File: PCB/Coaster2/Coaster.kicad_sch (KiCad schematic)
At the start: 409 parts

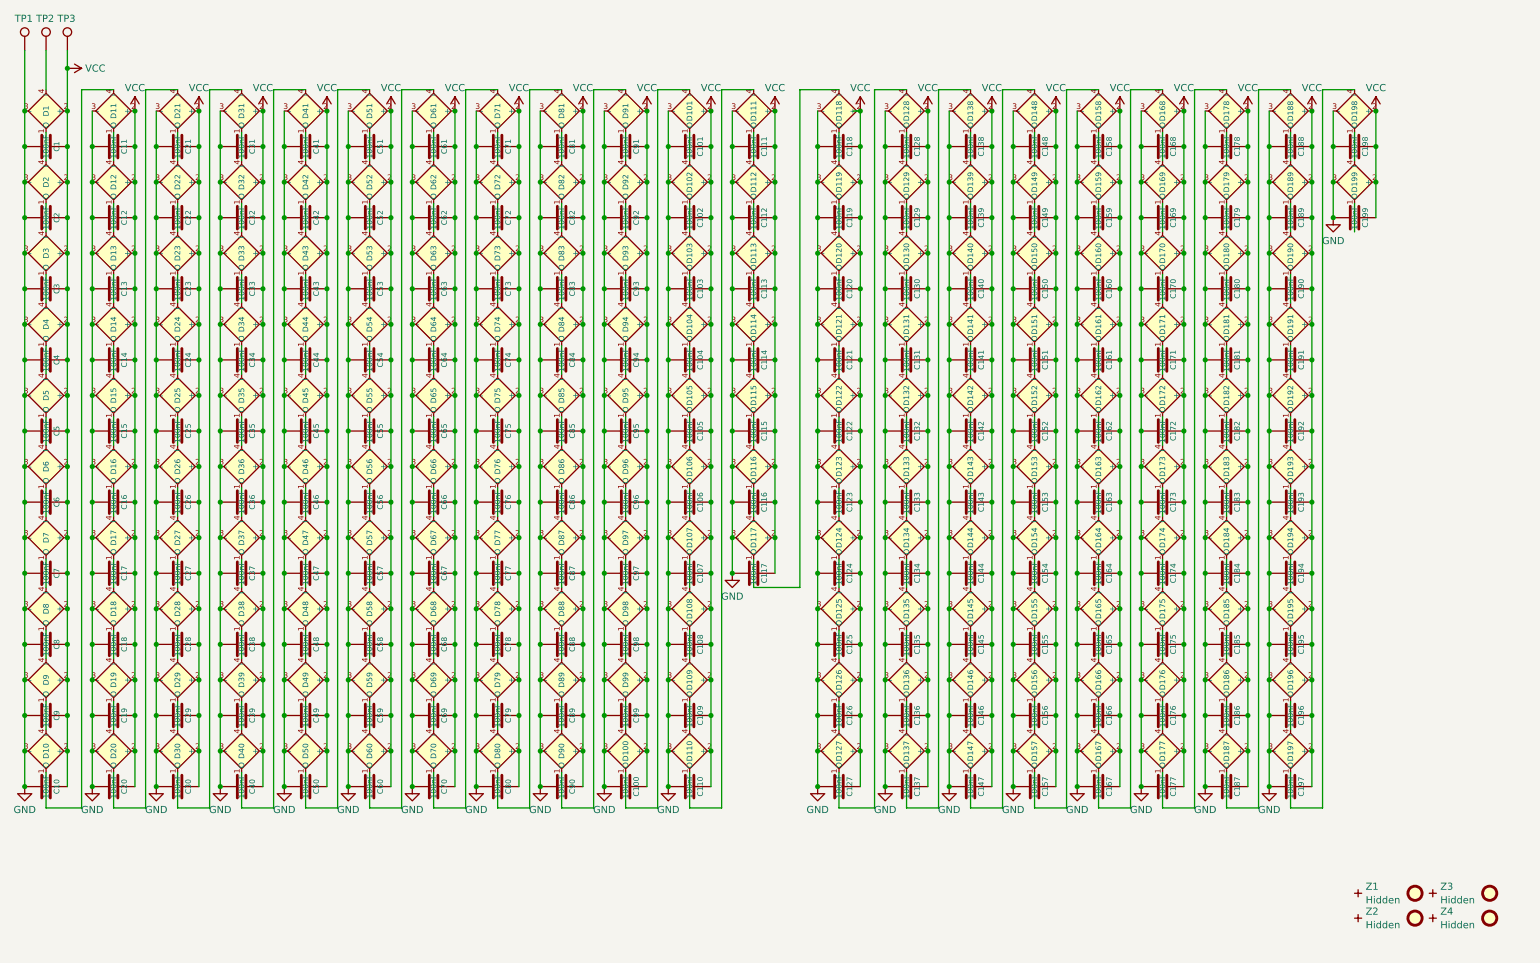
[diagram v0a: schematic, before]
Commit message: Tracked
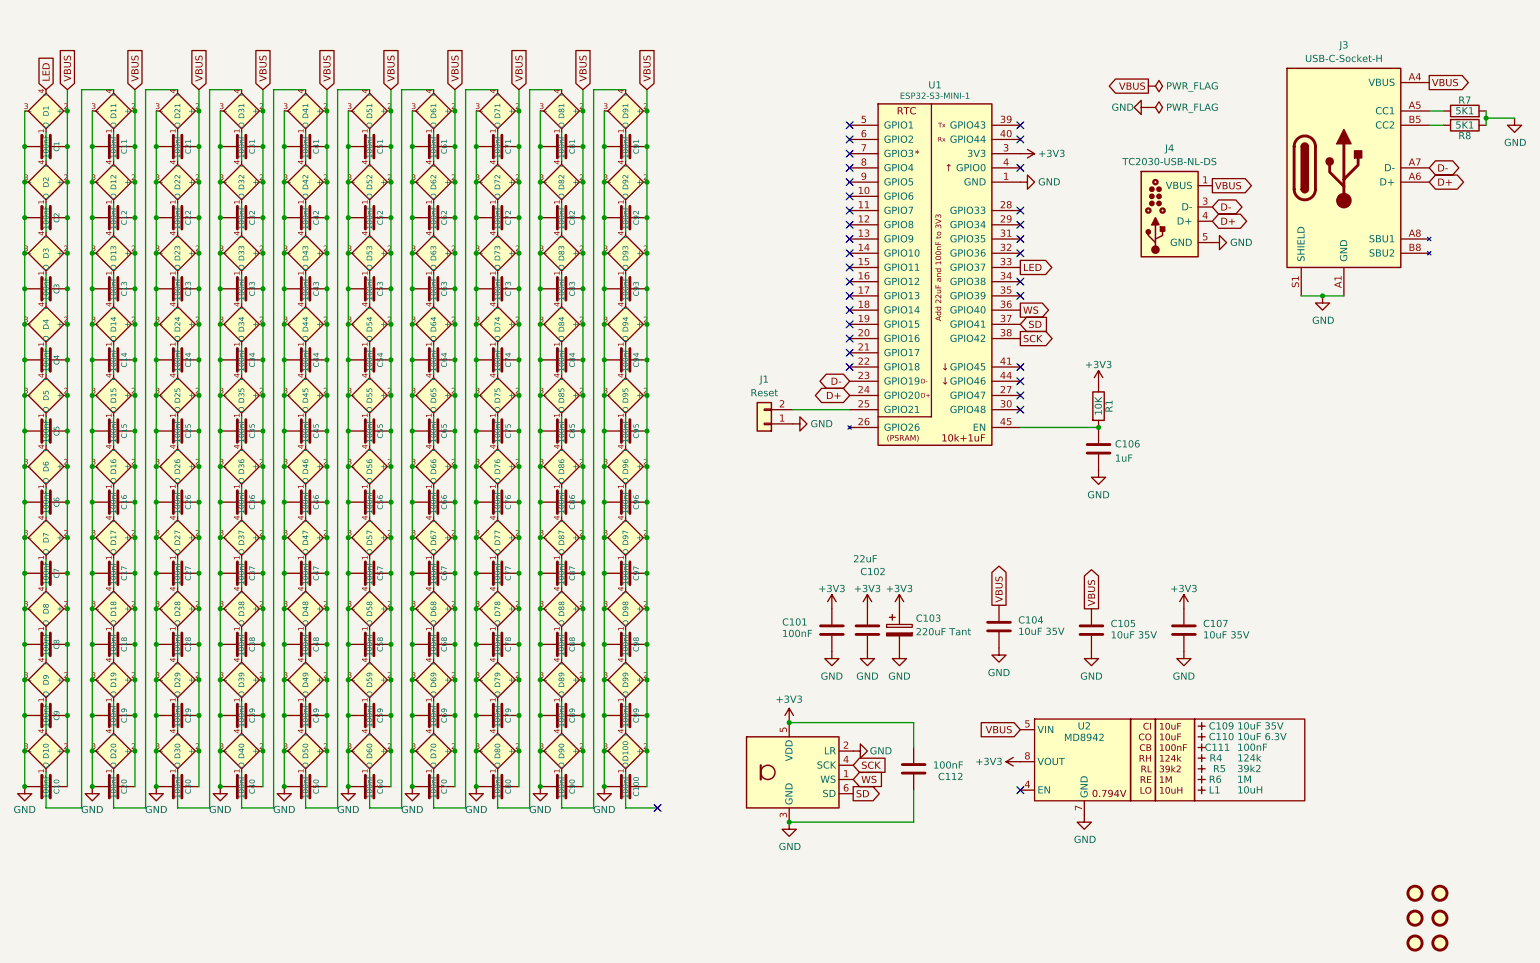
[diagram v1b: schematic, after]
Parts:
- removed C103, C108, C109, C110, C111, C113, C114, C115, C116, C117, C118, C119, C120, C121, C122, C123, C124, C125, C126, C127, C128, C129, C130, C131, C132, C133, C134, C135, C136, C137, C138, C139, C140, C141, C142, C143, C144, C145, C146, C147, C148, C149, C150, C151, C152, C153, C154, C155, C156, C157, C158, C159, C160, C161, C162, C163, C164, C165, C166, C167, C168, C169, C170, C171, C172, C173, C174, C175, C176, C177, C178, C179, C180, C181, C182, C183, C184, C185, C186, C187, C188, C189, C190, C191, C192, C193, C194, C195, C196, C197, C198, C199: 100nF, RevK:C_0402, symbol Device:C
- removed D101, D102, D103, D104, D105, D106, D107, D108, D109, D110, D111, D112, D113, D114, D115, D116, D117, D118, D119, D120, D121, D122, D123, D124, D125, D126, D127, D128, D129, D130, D131, D132, D133, D134, D135, D136, D137, D138, D139, D140, D141, D142, D143, D144, D145, D146, D147, D148, D149, D150, D151, D152, D153, D154, D155, D156, D157, D158, D159, D160, D161, D162, D163, D164, D165, D166, D167, D168, D169, D170, D171, D172, D173, D174, D175, D176, D177, D178, D179, D180, D181, D182, D183, D184, D185, D186, D187, D188, D189, D190, D191, D192, D193, D194, D195, D196, D197, D198, D199: XL-1010RGBC-WS2812B, RevK:SMD1010, symbol RevK:WS2812B-1mm
- removed TP1: GND, RevK:Round, symbol Connector:TestPoint
- removed TP2: DIN, RevK:Round, symbol Connector:TestPoint
- removed TP3: PWR, RevK:Round, symbol Connector:TestPoint
- removed Z1, Z2, Z3, Z4: Hidden, RevK:PCB-Join1, symbol RevK:Hidden
- added C103: 220uF Tant, RevK:CP_EIA-3528-21_Kemet-B, symbol Device:C_Polarized
- added C109: 10uF 35V, RevK:C_0603_, symbol RevK:Hidden
- added C110: 10uF 6.3V, RevK:C_0603_, symbol RevK:Hidden
- added C111: 100nF, RevK:C_0603_, symbol RevK:Hidden
- added FID5: Fiducial, RevK:Hole-Tooling, symbol Mechanical:Fiducial
- added FID6: Fiducial, Fiducial:Fiducial_1mm_Mask2mm, symbol Mechanical:Fiducial
- added J1: Reset, RevK:AA-Pad, symbol Connector_Generic:Conn_01x02
- added J3: USB-C-Socket-H, RevK:USB-C-Socket-H, symbol RevK:USB-C-Socket-H
- added J4: TC2030-USB-NL-DS, RevK:Tag-Connect_TC2030-IDC-NL_2x03_P1.27mm_Vertical, symbol RevK:TC2030-USB-NL
- added L1: 10uH, RevK:L_4x4_, symbol RevK:Hidden
- added R1: 10K, RevK:R_0402, symbol Device:R
- added R4: 124k, RevK:R_0402_, symbol RevK:Hidden
- added R5: 39k2, RevK:R_0402_, symbol RevK:Hidden
- added R6: 1M, RevK:R_0402_, symbol RevK:Hidden
- added R7, R8: 5K1, RevK:R_0402, symbol Device:R
- added U1: ESP32-S3-MINI-1, RevK:ESP32-S3-MINI-1, symbol RevK:ESP32-S3-MINI-1-N4R2
- added U2: MD8942, RevK:SOT-23-6-MD8942, symbol RevK:MD89420-RegBlock
- added U3: ICS43434_MEMS_Mic, RevK:ICS43434_MEMS_Mic, symbol RevK:ICS43434_MEMS_Mic
- C102: value 100nF -> 22uF; footprint RevK:C_0402 -> RevK:C_0603
- C104, C105, C107: value 100nF -> 10uF 35V; footprint RevK:C_0402 -> RevK:C_0603; LCSC Part # (none) -> C194427
- C106: value 100nF -> 1uF
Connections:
- net GND: now also C112.1, C103.2, J1.1 (Pin_1), J3.A1 (GND), J3.A12 (GND), J3.B1 (GND), J3.B12 (GND), J3.S1 (SHIELD), J4.5 (GND), J4.6 (GND), R7.2, R8.1, U1.1 (GND), U1.2 (GND), U1.42 (GND), U1.43 (GND), U1.46 (GND), U1.47 (GND), U1.48 (GND), U1.49 (GND), U1.50 (GND), U1.51 (GND), U1.52 (GND), U1.53 (GND), U1.54 (GND), U1.55 (GND), U1.56 (GND), U1.57 (GND), U1.58 (GND), U1.59 (GND), U1.60 (GND), U1.61 (GND), U1.62 (GND), U1.63 (GND), U1.64 (GND), U1.65 (GND), U2.2 (GND), U2.7 (GND), U3.2 (LR), U3.3 (GND); no longer C112.2
- net LED: now reaches D1.4 (I)
- net LED: now also U1.33 (GPIO37)
- net VCC renamed VBUS
- net VBUS: now also J3.A4 (VBUS), J3.A9 (VBUS), J3.B4 (VBUS), J3.B9 (VBUS), J4.1 (VBUS), J4.2 (VBUS), U2.5 (VIN); no longer C101.1, C102.1, C106.1, C107.1, C112.1
- new net: J3.A5 (CC1), R7.1
- new net: C106.1, R1.2, U1.45 (EN)
- new net: J3.B5 (CC2), R8.2
- new net: J1.2 (Pin_2), U1.25 (GPIO21)
- new net +3V3: C101.1, C102.1, C103.1, C107.1, C112.2, R1.1, U1.3 (3V3), U2.8 (VOUT), U3.5 (VDD)
- new net D+: J3.A6 (D+), J3.B6 (D+), J4.4 (D+), U1.24 (GPIO20)
- new net D-: J3.A7 (D-), J3.B7 (D-), J4.3 (D-), U1.23 (GPIO19)
- new net SCK: U1.38 (GPIO42), U3.4 (SCK)
- new net SD: U1.37 (GPIO41), U3.6 (SD)
- new net WS: U1.36 (GPIO40), U3.1 (WS)
- no-connect marks 0 -> 33

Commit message: 124 LEDs
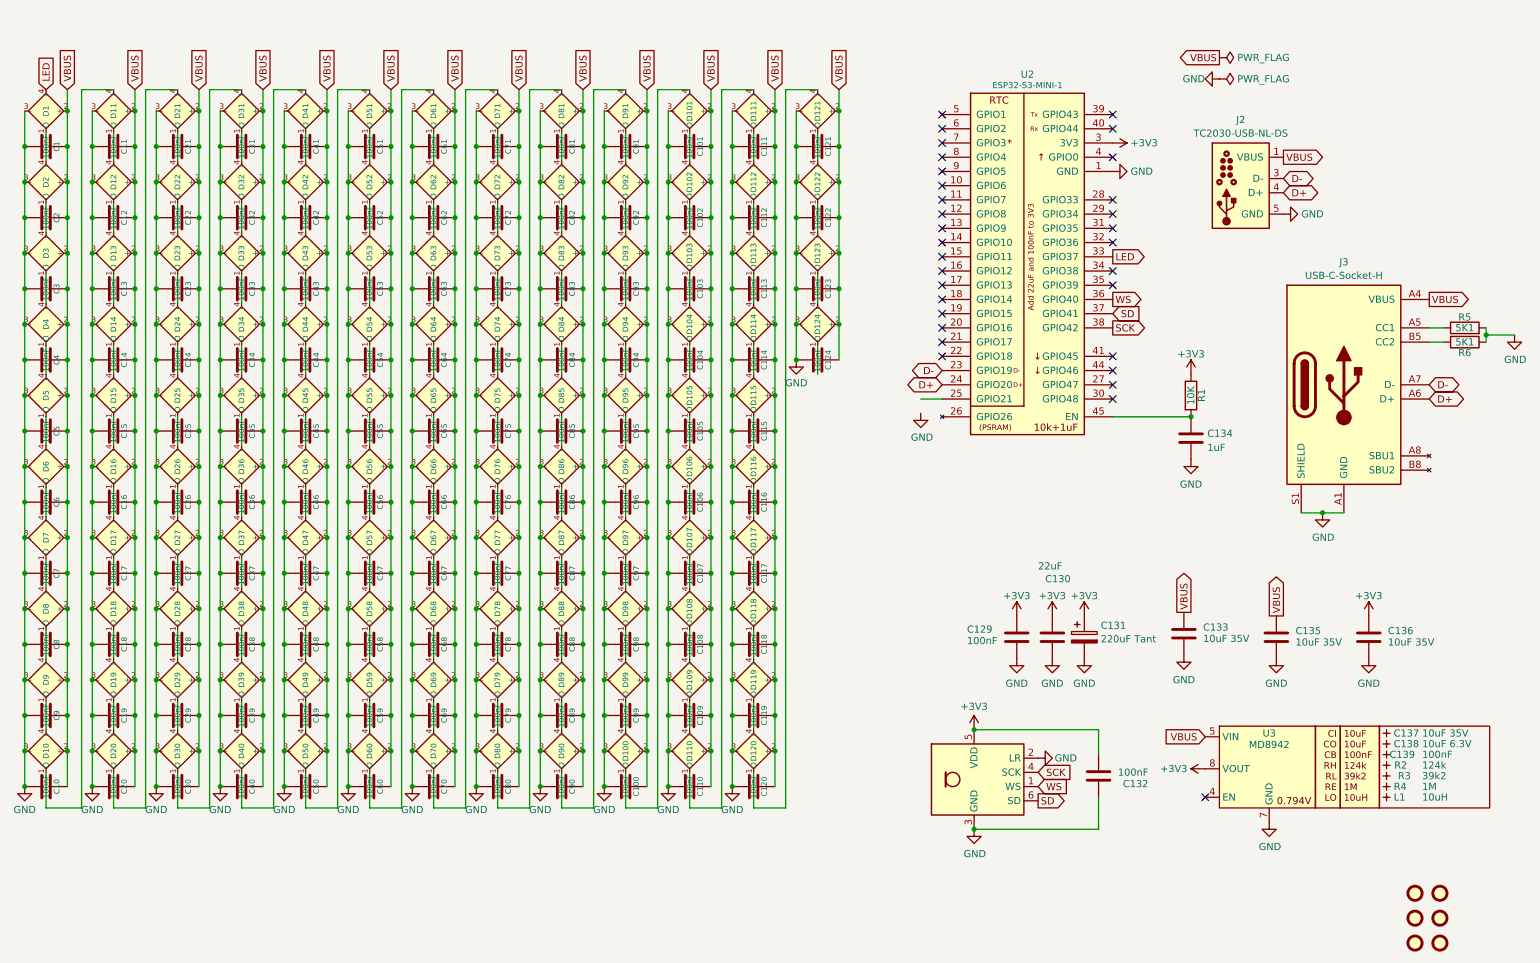
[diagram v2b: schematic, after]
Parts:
- removed J1: Reset, RevK:AA-Pad, symbol Connector_Generic:Conn_01x02
- added C101, C102, C103, C104, C105, C106, C107, C108, C109, C110, C111, C112, C113, C114, C115, C116, C117, C118, C119, C120, C121, C122, C123, C124: 100nF, RevK:C_0402, symbol Device:C
- added D101, D102, D103, D104, D105, D106, D107, D108, D109, D110, D111, D112, D113, D114, D115, D116, D117, D118, D119, D120, D121, D122, D123, D124: XL-1010RGBC-WS2812B, RevK:SMD1010, symbol RevK:WS2812B-1mm
- renumbered C101 to C129, C102 to C130, C103 to C131, C112 to C132, C104 to C133, C106 to C134, C105 to C135, C107 to C136, C109 to C137, C110 to C138, C111 to C139, FID5 to FID1, FID4 to FID3, FID6 to FID4, FID1 to FID5, FID3 to FID6, J4 to J2, R4 to R2, R5 to R3, R6 to R4, R7 to R5, R8 to R6, U3 to U1, U1 to U2, U2 to U3
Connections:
- net GND: now also C101.2, C102.2, C103.2, C104.2, C105.2, C106.2, C107.2, C108.2, C109.2, C110.2, C111.2, C112.2, C113.2, C114.2, C115.2, C116.2, C117.2, C118.2, C119.2, C120.2, C121.2, C122.2, C123.2, C124.2, D101.3 (-), D102.3 (-), D103.3 (-), D104.3 (-), D105.3 (-), D106.3 (-), D107.3 (-), D108.3 (-), D109.3 (-), D110.3 (-), D111.3 (-), D112.3 (-), D113.3 (-), D114.3 (-), D115.3 (-), D116.3 (-), D117.3 (-), D118.3 (-), D119.3 (-), D120.3 (-), D121.3 (-), D122.3 (-), D123.3 (-), D124.3 (-)
- net VBUS: now also C101.1, C102.1, C103.1, C104.1, C105.1, C106.1, C107.1, C108.1, C109.1, C110.1, C111.1, C112.1, C113.1, C114.1, C115.1, C116.1, C117.1, C118.1, C119.1, C120.1, C121.1, C122.1, C123.1, C124.1, D101.2 (+), D102.2 (+), D103.2 (+), D104.2 (+), D105.2 (+), D106.2 (+), D107.2 (+), D108.2 (+), D109.2 (+), D110.2 (+), D111.2 (+), D112.2 (+), D113.2 (+), D114.2 (+), D115.2 (+), D116.2 (+), D117.2 (+), D118.2 (+), D119.2 (+), D120.2 (+), D121.2 (+), D122.2 (+), D123.2 (+), D124.2 (+)
- net at D100.1 (O): now also D101.4 (I)
- new net: D117.1 (O), D118.4 (I)
- new net: D116.1 (O), D117.4 (I)
- new net: D109.1 (O), D110.4 (I)
- new net: D108.1 (O), D109.4 (I)
- new net: D115.1 (O), D116.4 (I)
- new net: D121.1 (O), D122.4 (I)
- new net: D120.1 (O), D121.4 (I)
- new net: D113.1 (O), D114.4 (I)
- new net: D112.1 (O), D113.4 (I)
- new net: D104.1 (O), D105.4 (I)
- new net: D103.1 (O), D104.4 (I)
- new net: D107.1 (O), D108.4 (I)
- new net: D102.1 (O), D103.4 (I)
- new net: D110.1 (O), D111.4 (I)
- new net: D114.1 (O), D115.4 (I)
- new net: D123.1 (O), D124.4 (I)
- new net: D101.1 (O), D102.4 (I)
- new net: D111.1 (O), D112.4 (I)
- new net: D119.1 (O), D120.4 (I)
- new net: D118.1 (O), D119.4 (I)
- new net: D122.1 (O), D123.4 (I)
- new net: D106.1 (O), D107.4 (I)
- new net: D105.1 (O), D106.4 (I)
- no-connect marks 33 -> 32
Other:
- moved on the sheet: C129, C130, C131, C132, C133, C134, C135, C136, C137, C138, C139, J2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
